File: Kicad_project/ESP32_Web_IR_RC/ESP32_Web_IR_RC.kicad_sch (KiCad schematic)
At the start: 8 parts, among them J1 Trigger_input, J2 IR_output, U1 PC817

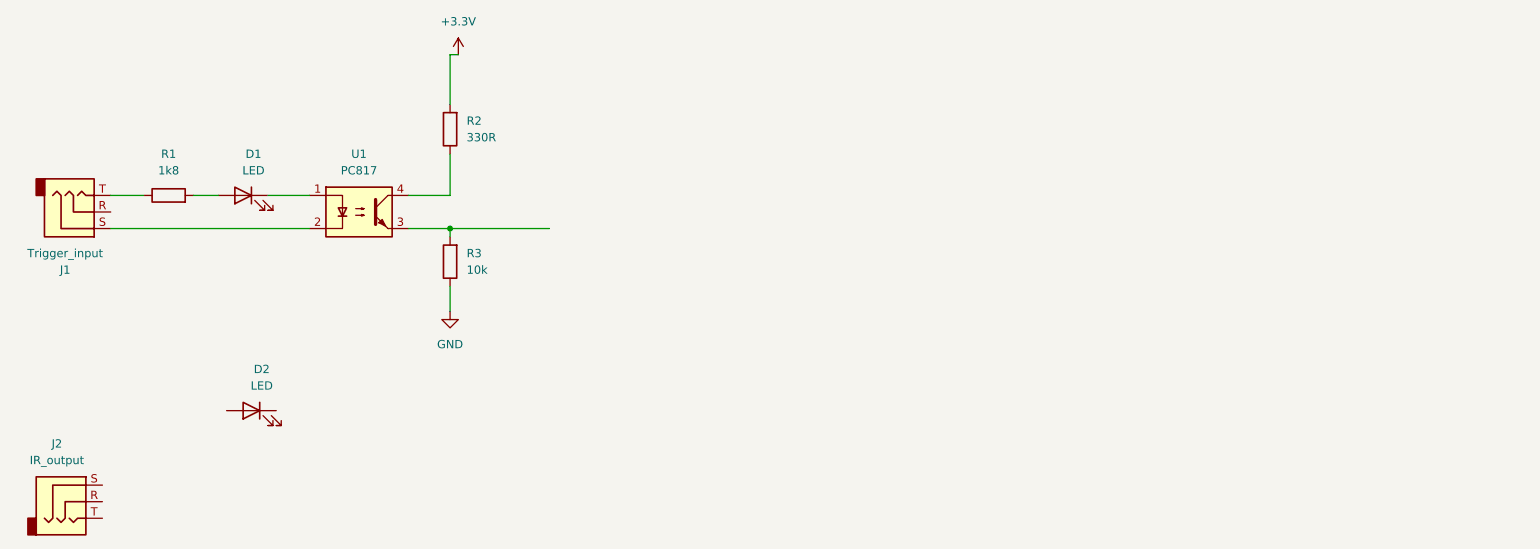
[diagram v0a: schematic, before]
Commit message: update
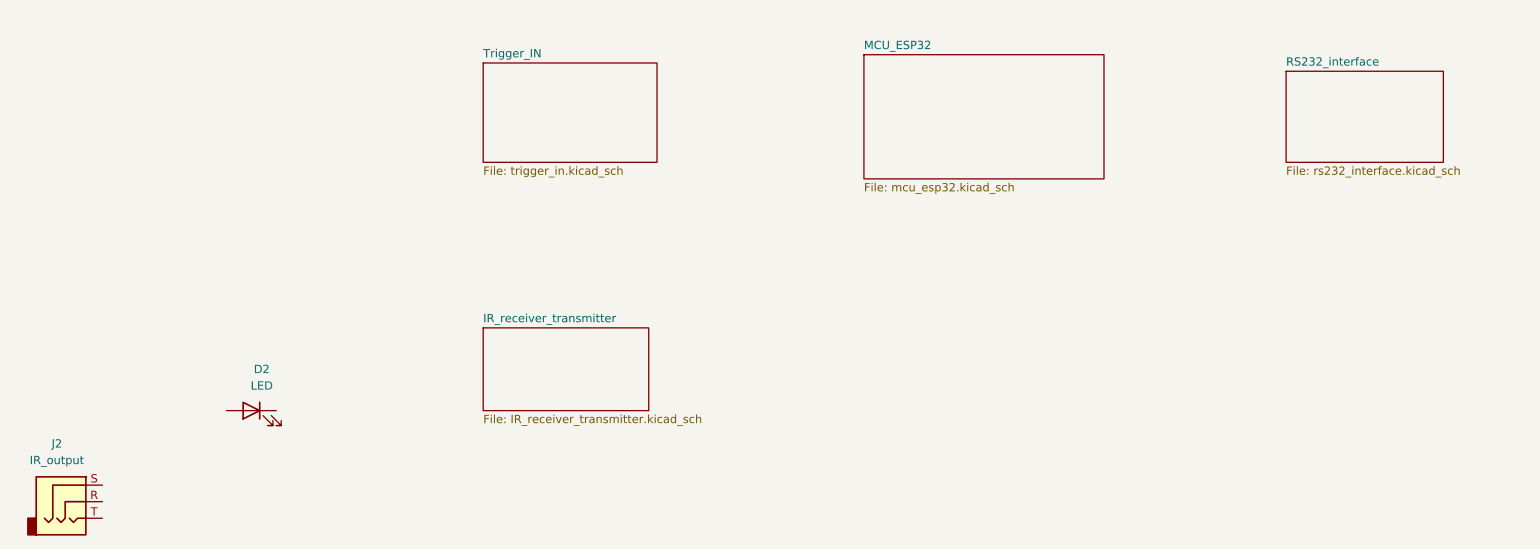
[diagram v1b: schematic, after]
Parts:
- removed D1: LED, symbol Device:LED
- removed J1: Trigger_input, Connector_Audio:Jack_3.5mm_CUI_SJ-3523-SMT_Horizontal, symbol Connector_Audio:AudioJack3
- removed R1: 1k8, Resistor_SMD:R_0805_2012Metric, symbol Device:R
- removed R2: 330R, Resistor_SMD:R_0805_2012Metric, symbol Device:R
- removed R3: 10k, Resistor_SMD:R_0805_2012Metric, symbol Device:R
- removed U1: PC817, Package_DIP:DIP-4_W7.62mm, symbol Isolator:PC817
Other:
- added sheet IR_receiver_transmitter (IR_receiver_transmitter.kicad_sch)
- added sheet MCU_ESP32 (mcu_esp32.kicad_sch)
- added sheet RS232_interface (rs232_interface.kicad_sch)
- added sheet Trigger_IN (trigger_in.kicad_sch)
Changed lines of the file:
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@@
 (kicad_sch (version 20230121) (generator eeschema)
   (paper "A4")
-  (junction (at 104.14 60.96) (diameter 0) (color 0 0 0 0)
-  )
-  (wire (pts (xy 104.14 60.96) (xy 104.14 62.23))
-    (stroke (width 0) (type default))
-  )
-  (wire (pts (xy 104.14 55.88) (xy 97.79 55.88))
-    (stroke (width 0) (type default))
-  )
-  (wire (pts (xy 104.14 34.29) (xy 105.41 34.29))
-    (stroke (width 0) (type default))
-  )
-  (wire (pts (xy 52.07 55.88) (xy 57.15 55.88))
-    (stroke (width 0) (type default))
-  )
-  (wire (pts (xy 104.14 49.53) (xy 104.14 55.88))
-    (stroke (width 0) (type default))
-  )
-  (wire (pts (xy 76.2 55.88) (xy 82.55 55.88))
-    (stroke (width 0) (type default))
-  )
-  (wire (pts (xy 64.77 55.88) (xy 68.58 55.88))
-    (stroke (width 0) (type default))
-  )
-  (wire (pts (xy 97.79 60.96) (xy 104.14 60.96))
-    (stroke (width 0) (type default))
-  )
-  (wire (pts (xy 104.14 69.85) (xy 104.14 73.66))
-    (stroke (width 0) (type default))
-  )
-  (wire (pts (xy 52.07 60.96) (xy 82.55 60.96))
-    (stroke (width 0) (type default))
-  )
-  (wire (pts (xy 104.14 41.91) (xy 104.14 34.29))
-    (stroke (width 0) (type default))
-  )
-  (wire (pts (xy 104.14 60.96) (xy 119.38 60.96))
-    (stroke (width 0) (type default))
-  )
   (symbol (lib_id "Connector_Audio:AudioJack3") (at 45.72 102.87 0) (unit 1)
     (in_bom yes) (on_board yes) (dnp no) (fields_autoplaced)
@@
         (path "/eff9f25b-fc22-435c-ba15-64107809273b"
           (reference "J2") (unit 1)
-        )
-      )
-    )
-  )
-  (symbol (lib_id "Device:R") (at 104.14 45.72 180) (unit 1)
-    (in_bom yes) (on_board yes) (dnp no) (fields_autoplaced)
-    (property "Reference" "R2" (at 106.68 44.45 0)
-      (effects (font (size 1.27 1.27)) (justify right))
-    )
-    (property "Value" "330R" (at 106.68 46.99 0)
-      (effects (font (size 1.27 1.27)) (justify right))
-    )
-    (property "Footprint" "Resistor_SMD:R_0805_2012Metric" (at 105.918 45.72 90)
-      (effects (font (size 1.27 1.27)) hide)
-    )
-    (property "Datasheet" "~" (at 104.14 45.72 0)
-      (effects (font (size 1.27 1.27)) hide)
-    )
-    (pin "2")
-    (pin "1")
-    (instances
-      (project "ESP32_Web_IR_RC"
-        (path "/eff9f25b-fc22-435c-ba15-64107809273b"
-          (reference "R2") (unit 1)
-        )
-      )
-    )
-  )
-  (symbol (lib_id "power:GND") (at 104.14 73.66 0) (unit 1)
-    (in_bom yes) (on_board yes) (dnp no) (fields_autoplaced)
-    (property "Reference" "#PWR02" (at 104.14 80.01 0)
-      (effects (font (size 1.27 1.27)) hide)
-    )
-    (property "Value" "GND" (at 104.14 78.74 0)
-      (effects (font (size 1.27 1.27)))
-    )
-    (property "Footprint" "" (at 104.14 73.66 0)
-      (effects (font (size 1.27 1.27)) hide)
-    )
-    (property "Datasheet" "" (at 104.14 73.66 0)
-      (effects (font (size 1.27 1.27)) hide)
-    )
-    (pin "1")
-    (instances
-      (project "ESP32_Web_IR_RC"
-        (path "/eff9f25b-fc22-435c-ba15-64107809273b"
-          (reference "#PWR02") (unit 1)
-        )
-      )
-    )
-  )
-  (symbol (lib_id "Device:LED") (at 72.39 55.88 0) (mirror y) (unit 1)
-    (in_bom yes) (on_board yes) (dnp no)
-    (property "Reference" "D1" (at 73.9775 49.53 0)
-      (effects (font (size 1.27 1.27)))
-    )
-    (property "Value" "LED" (at 73.9775 52.07 0)
-      (effects (font (size 1.27 1.27)))
-    )
-    (property "Footprint" "" (at 72.39 55.88 0)
-      (effects (font (size 1.27 1.27)) hide)
-    )
-    (property "Datasheet" "~" (at 72.39 55.88 0)
-      (effects (font (size 1.27 1.27)) hide)
-    )
-    (pin "2")
-    (pin "1")
-    (instances
-      (project "ESP32_Web_IR_RC"
-        (path "/eff9f25b-fc22-435c-ba15-64107809273b"
-          (reference "D1") (unit 1)
-        )
-      )
-    )
-  )
-  (symbol (lib_id "Device:R") (at 104.14 66.04 180) (unit 1)
-    (in_bom yes) (on_board yes) (dnp no) (fields_autoplaced)
-    (property "Reference" "R3" (at 106.68 64.77 0)
-      (effects (font (size 1.27 1.27)) (justify right))
-    )
-    (property "Value" "10k" (at 106.68 67.31 0)
-      (effects (font (size 1.27 1.27)) (justify right))
-    )
-    (property "Footprint" "Resistor_SMD:R_0805_2012Metric" (at 105.918 66.04 90)
-      (effects (font (size 1.27 1.27)) hide)
-    )
-    (property "Datasheet" "~" (at 104.14 66.04 0)
-      (effects (font (size 1.27 1.27)) hide)
-    )
-    (pin "2")
-    (pin "1")
-    (instances
-      (project "ESP32_Web_IR_RC"
-        (path "/eff9f25b-fc22-435c-ba15-64107809273b"
-          (reference "R3") (unit 1)
-        )
-      )
-    )
-  )
-  (symbol (lib_id "power:+3.3V") (at 105.41 34.29 0) (unit 1)
-    (in_bom yes) (on_board yes) (dnp no) (fields_autoplaced)
-    (property "Reference" "#PWR01" (at 105.41 38.1 0)
-      (effects (font (size 1.27 1.27)) hide)
-    )
-    (property "Value" "+3.3V" (at 105.41 29.21 0)
-      (effects (font (size 1.27 1.27)))
-    )
-    (property "Footprint" "" (at 105.41 34.29 0)
-      (effects (font (size 1.27 1.27)) hide)
-    )
-    (property "Datasheet" "" (at 105.41 34.29 0)
-      (effects (font (size 1.27 1.27)) hide)
-    )
-    (pin "1")
-    (instances
-      (project "ESP32_Web_IR_RC"
-        (path "/eff9f25b-fc22-435c-ba15-64107809273b"
-          (reference "#PWR01") (unit 1)
-        )
-      )
-    )
-  )
-  (symbol (lib_id "Device:R") (at 60.96 55.88 90) (unit 1)
-    (in_bom yes) (on_board yes) (dnp no) (fields_autoplaced)
-    (property "Reference" "R1" (at 60.96 49.53 90)
-      (effects (font (size 1.27 1.27)))
-    )
-    (property "Value" "1k8" (at 60.96 52.07 90)
-      (effects (font (size 1.27 1.27)))
-    )
-    (property "Footprint" "Resistor_SMD:R_0805_2012Metric" (at 60.96 57.658 90)
-      (effects (font (size 1.27 1.27)) hide)
-    )
-    (property "Datasheet" "~" (at 60.96 55.88 0)
-      (effects (font (size 1.27 1.27)) hide)
-    )
-    (pin "2")
-    (pin "1")
-    (instances
-      (project "ESP32_Web_IR_RC"
-        (path "/eff9f25b-fc22-435c-ba15-64107809273b"
-          (reference "R1") (unit 1)
-        )
-      )
-    )
-  )
-  (symbol (lib_id "Isolator:PC817") (at 90.17 58.42 0) (unit 1)
-    (in_bom yes) (on_board yes) (dnp no) (fields_autoplaced)
-    (property "Reference" "U1" (at 90.17 49.53 0)
-      (effects (font (size 1.27 1.27)))
-    )
-    (property "Value" "PC817" (at 90.17 52.07 0)
-      (effects (font (size 1.27 1.27)))
-    )
-    (property "Footprint" "Package_DIP:DIP-4_W7.62mm" (at 85.09 63.5 0)
-      (effects (font (size 1.27 1.27) italic) (justify left) hide)
-    )
-    (property "Datasheet" "http://www.soselectronic.cz/a_info/resource/d/pc817.pdf" (at 90.17 58.42 0)
-      (effects (font (size 1.27 1.27)) (justify left) hide)
-    )
-    (pin "2")
-    (pin "3")
-    (pin "1")
-    (pin "4")
-    (instances
-      (project "ESP32_Web_IR_RC"
-        (path "/eff9f25b-fc22-435c-ba15-64107809273b"
-          (reference "U1") (unit 1)
         )
       )
@@
     )
   )
-  (symbol (lib_id "Connector_Audio:AudioJack3") (at 46.99 58.42 0) (mirror x) (unit 1)
-    (in_bom yes) (on_board yes) (dnp no)
-    (property "Reference" "J1" (at 45.085 67.31 0)
-      (effects (font (size 1.27 1.27)))
+  (sheet (at 109.22 35.56) (size 26.67 15.24) (fields_autoplaced)
+    (stroke (width 0.1524) (type solid))
+    (fill (color 0 0 0 0.0000))
+    (property "Sheetname" "Trigger_IN" (at 109.22 34.8484 0)
+      (effects (font (size 1.27 1.27)) (justify left bottom))
     )
-    (property "Value" "Trigger_input" (at 45.085 64.77 0)
-      (effects (font (size 1.27 1.27)))
+    (property "Sheetfile" "trigger_in.kicad_sch" (at 109.22 51.3846 0)
+      (effects (font (size 1.27 1.27)) (justify left top))
     )
-    (property "Footprint" "Connector_Audio:Jack_3.5mm_CUI_SJ-3523-SMT_Horizontal" (at 46.99 58.42 0)
-      (effects (font (size 1.27 1.27)) hide)
-    )
-    (property "Datasheet" "~" (at 46.99 58.42 0)
-      (effects (font (size 1.27 1.27)) hide)
-    )
-    (pin "S")
-    (pin "R")
-    (pin "T")
     (instances
       (project "ESP32_Web_IR_RC"
-        (path "/eff9f25b-fc22-435c-ba15-64107809273b"
-          (reference "J1") (unit 1)
-        )
+        (path "/eff9f25b-fc22-435c-ba15-64107809273b" (page "2"))
       )
     )
+  )
+  (sheet (at 232.41 36.83) (size 24.13 13.97) (fields_autoplaced)
+    (stroke (width 0.1524) (type solid))
+    (fill (color 0 0 0 0.0000))
+    (property "Sheetname" "RS232_interface" (at 232.41 36.1184 0)
+      (effects (font (size 1.27 1.27)) (justify left bottom))
+    )
+    (property "Sheetfile" "rs232_interface.kicad_sch" (at 232.41 51.3846 0)
+      (effects (font (size 1.27 1.27)) (justify left top))
+    )
+    (instances
+      (project "ESP32_Web_IR_RC"
+        (path "/eff9f25b-fc22-435c-ba15-64107809273b" (page "4"))
+      )
+    )
+  )
+  (sheet (at 167.64 34.29) (size 36.83 19.05) (fields_autoplaced)
+    (stroke (width 0.1524) (type solid))
+    (fill (color 0 0 0 0.0000))
+    (property "Sheetname" "MCU_ESP32" (at 167.64 33.5784 0)
+      (effects (font (size 1.27 1.27)) (justify left bottom))
+    )
+    (property "Sheetfile" "mcu_esp32.kicad_sch" (at 167.64 53.9246 0)
+      (effects (font (size 1.27 1.27)) (justify left top))
+    )
+    (instances
+      (project "ESP32_Web_IR_RC"
+        (path "/eff9f25b-fc22-435c-ba15-64107809273b" (page "5"))
+      )
+    )
+  )
+  (sheet (at 109.22 76.2) (size 25.4 12.7) (fields_autoplaced)
+    (stroke (width 0.1524) (type solid))
+    (fill (color 0 0 0 0.0000))
+    (property "Sheetname" "IR_receiver_transmitter" (at 109.22 75.4884 0)
+      (effects (font (size 1.27 1.27)) (justify left bottom))
+    )
+    (property "Sheetfile" "IR_receiver_transmitter.kicad_sch" (at 109.22 89.4846 0)
+      (effects (font (size 1.27 1.27)) (justify left top))
+    )
+    (instances
+      (project "ESP32_Web_IR_RC"
+        (path "/eff9f25b-fc22-435c-ba15-64107809273b" (page "3"))
+      )
+    )
